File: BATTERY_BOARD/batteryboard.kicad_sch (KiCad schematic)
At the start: 32 parts, among them J1 KEYSTONE-1042, J10 Screw_Terminal_01x02, J11 Screw_Terminal_01x02, J12 Screw_Terminal_01x01, J2 KEYSTONE-1042, J3 KEYSTONE-1042, J4 KEYSTONE-1042, J5 KEYSTONE-1042, J6 KEYSTONE-1042, J7 JST_PH_S2B-PH-SM4, J8 Screw_Terminal_01x02, J9 Screw_Terminal_01x02, Q1 IRF7458, Q2 IRF7458, U1 R5460N233AF

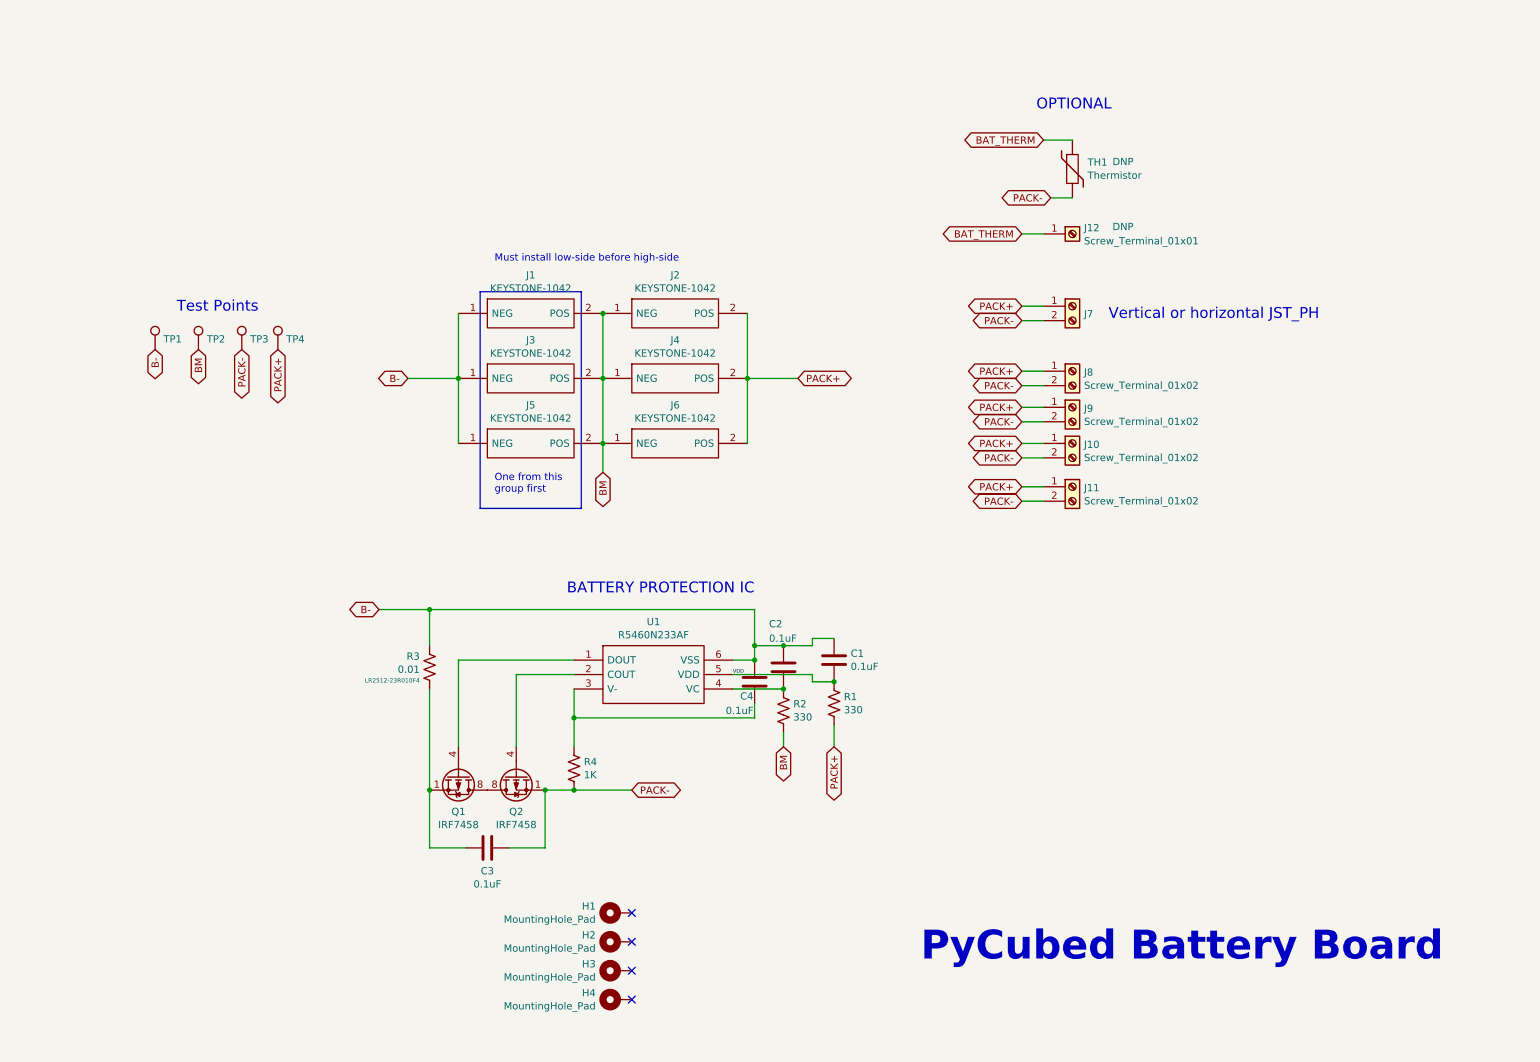
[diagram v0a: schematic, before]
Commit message: Battery Board Final Update
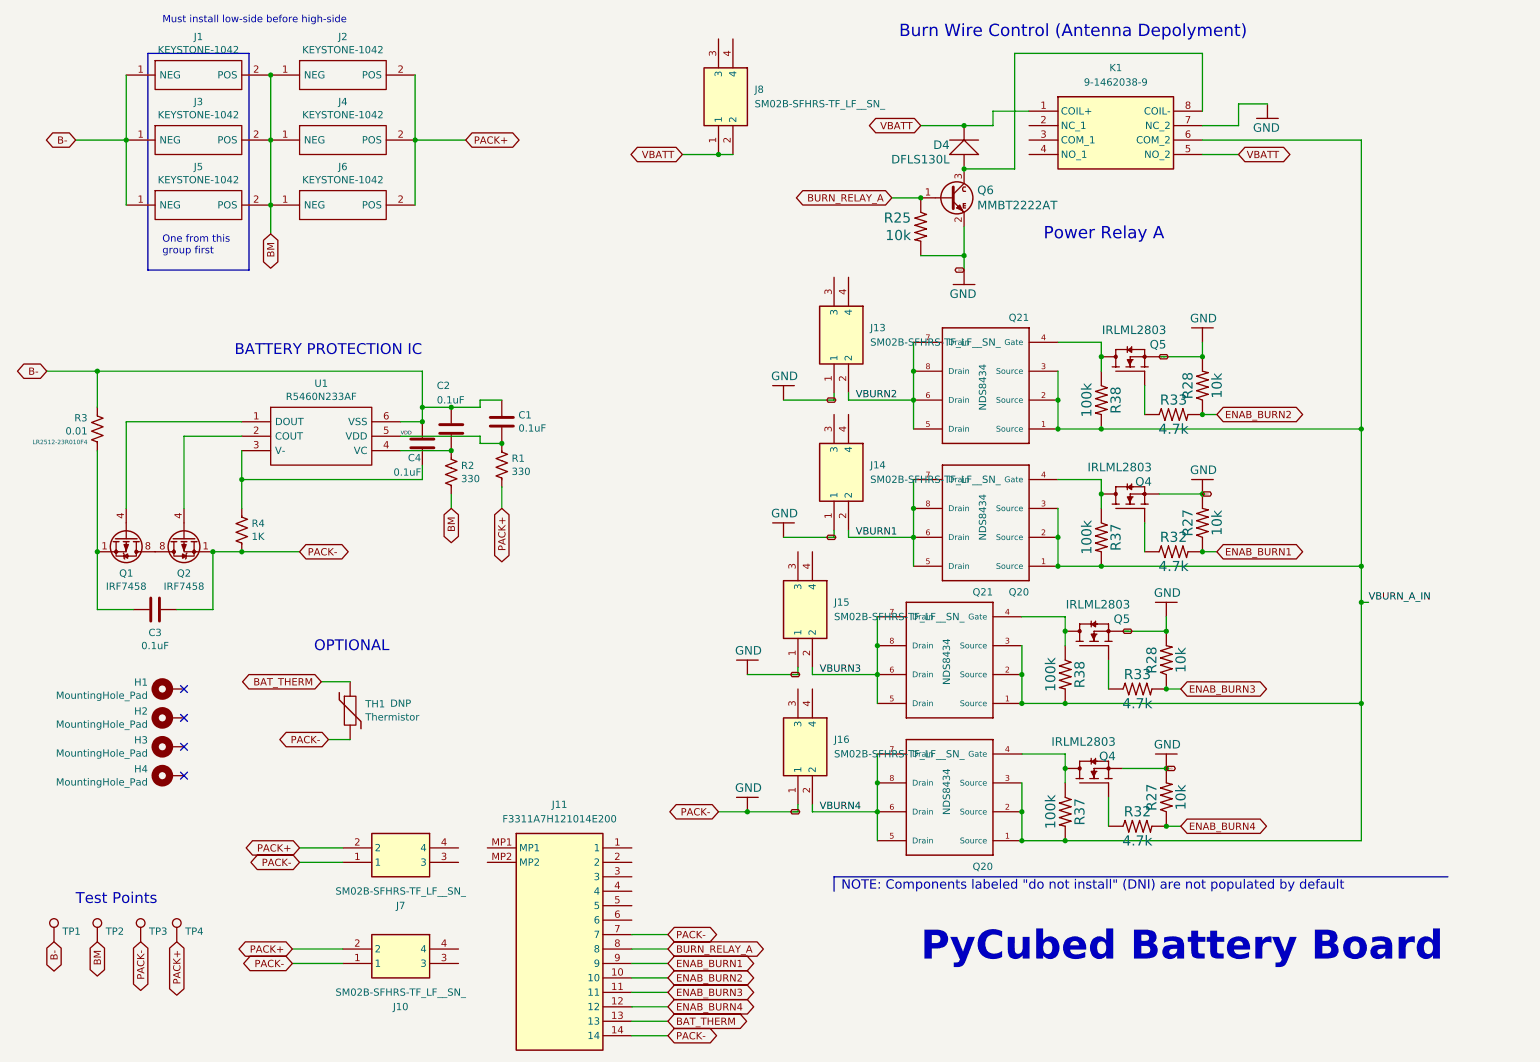
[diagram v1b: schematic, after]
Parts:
- removed J10, J11, J8, J9: Screw_Terminal_01x02, custom-footprints:SCREWTERMINAL-3.5MM-2_LOCK, symbol Connector:Screw_Terminal_01x02
- removed J12: Screw_Terminal_01x01, Connector_PinHeader_1.00mm:PinHeader_1x01_P1.00mm_Vertical, symbol Connector:Screw_Terminal_01x01
- removed J7: JST_PH_S2B-PH-SM4, Connector_JST:JST_PH_S2B-PH-SM4-TB_1x02-1MP_P2.00mm_Horizontal, symbol Connector:Screw_Terminal_01x02
- added D4: DFLS130L, mainboard:PWRDI-123, symbol mainboard:DFLS130L
- added J10, J13, J14, J15, J16, J7, J8: SM02B-SFHRS-TF_LF__SN_, SM02BSFHRSTFLFSN, symbol SamacSys_Parts:SM02B-SFHRS-TF_LF__SN_
- added J11: F3311A7H121014E200, F3311A7H121014E200, symbol SamacSys_Parts:F3311A7H121014E200
- added K1: 9-1462038-9, 914620389, symbol SamacSys_Parts:9-1462038-9
- added Q20 (x2), Q21 (x2): NDS8434, mainboard:NDS8434, symbol mainboard:NDS8434
- added Q4 (x2), Q5 (x2): IRLML2803, mainboard:SOT-23, symbol mainboard:IRLML2803TRPBF
- added Q6: MMBT2222AT, mainboard:SOT-23, symbol mainboard:MMBT2222AT
- added R25, R27 (x2), R28 (x2): 10k, Resistor_SMD:R_0603_1608Metric, symbol mainboard:RESISTOR0603
- added R32 (x2), R33 (x2): 4.7k, Resistor_SMD:R_0603_1608Metric, symbol mainboard:RESISTOR0603
- added R37 (x2), R38 (x2): 100k, Resistor_SMD:R_0603_1608Metric, symbol mainboard:RESISTOR0603
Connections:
- net BAT_THERM: now also J11.13
- net PACK+: now also J10.2, J7.2
- net PACK- renamed GND
- net GND: now also J10.1, J11.14, J11.7, J13.1, J14.1, J15.1, J16.1, J7.1, K1.7 (NC_2), Q4.2 (S), Q4.2 (S), Q5.2 (S), Q5.2 (S), Q6.2 (E), R25.2, R27.2, R27.2, R28.2, R28.2
- new net: D4.A, K1.8 (COIL-), Q6.3 (C)
- new net: Q20.4 (Gate), Q4.3 (D), R37.1 (x2)
- new net: Q21.4 (Gate), Q5.3 (D), R38.1 (x2)
- new net: Q5.1 (G), R33.1 (x2)
- new net: Q4.1 (G), R32.1 (x2)
- new net BURN_RELAY_A: J11.8, Q6.1 (B), R25.1
- new net ENAB_BURN1: J11.9, R27.1, R32.2
- new net ENAB_BURN2: J11.10, R28.1, R33.2
- new net ENAB_BURN3: J11.11, R28.1, R33.2
- new net ENAB_BURN4: J11.12, R27.1, R32.2
- new net VBATT: D4.C, J8.1, J8.2, K1.1 (COIL+), K1.5 (NO_2)
- new net VBURN1: J14.2, Q20.5 (Drain), Q20.6 (Drain), Q20.7 (Drain), Q20.8 (Drain)
- new net VBURN2: J13.2, Q21.5 (Drain), Q21.6 (Drain), Q21.7 (Drain), Q21.8 (Drain)
- new net VBURN3: J15.2, Q21.5 (Drain), Q21.6 (Drain), Q21.7 (Drain), Q21.8 (Drain)
- new net VBURN4: J16.2, Q20.5 (Drain), Q20.6 (Drain), Q20.7 (Drain), Q20.8 (Drain)
- new net VBURN_A_IN: K1.6 (COM_2), Q20.1 (Source), Q20.1 (Source), Q20.2 (Source), Q20.2 (Source), Q20.3 (Source), Q20.3 (Source), Q21.1 (Source), Q21.1 (Source), Q21.2 (Source), Q21.2 (Source), Q21.3 (Source), Q21.3 (Source), R37.2, R37.2, R38.2, R38.2
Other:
- note added: "Burn Wire Control (Antenna Depolyment)"
- note added: "NOTE: Components labeled "do not install" (DNI) are not populated by default"
- note added: "Power Relay A"
- note removed: "Vertical or horizontal JST_PH"
- moved on the sheet: C1, C2, C3, C4, H1, H2, H3, H4, J1, J2, J3, J4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
